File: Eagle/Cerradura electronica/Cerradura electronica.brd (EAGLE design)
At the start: 48.5 x 50 mm, 38 parts, among them IC1 LD117AS50TR, Q1 2N3904, Q2 IRF540NS, U1 ATMEGA328P_TQFP

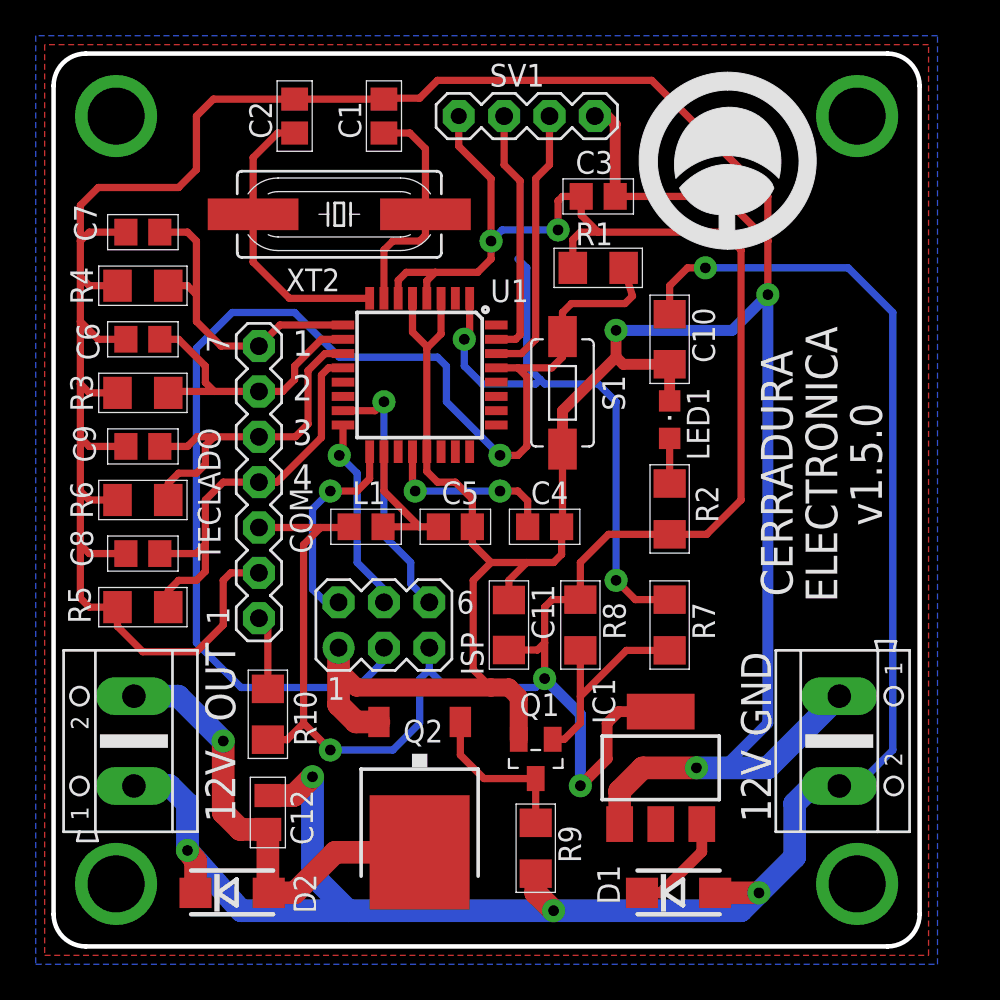
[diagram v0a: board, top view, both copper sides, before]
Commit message: Inicio correciones en PCB
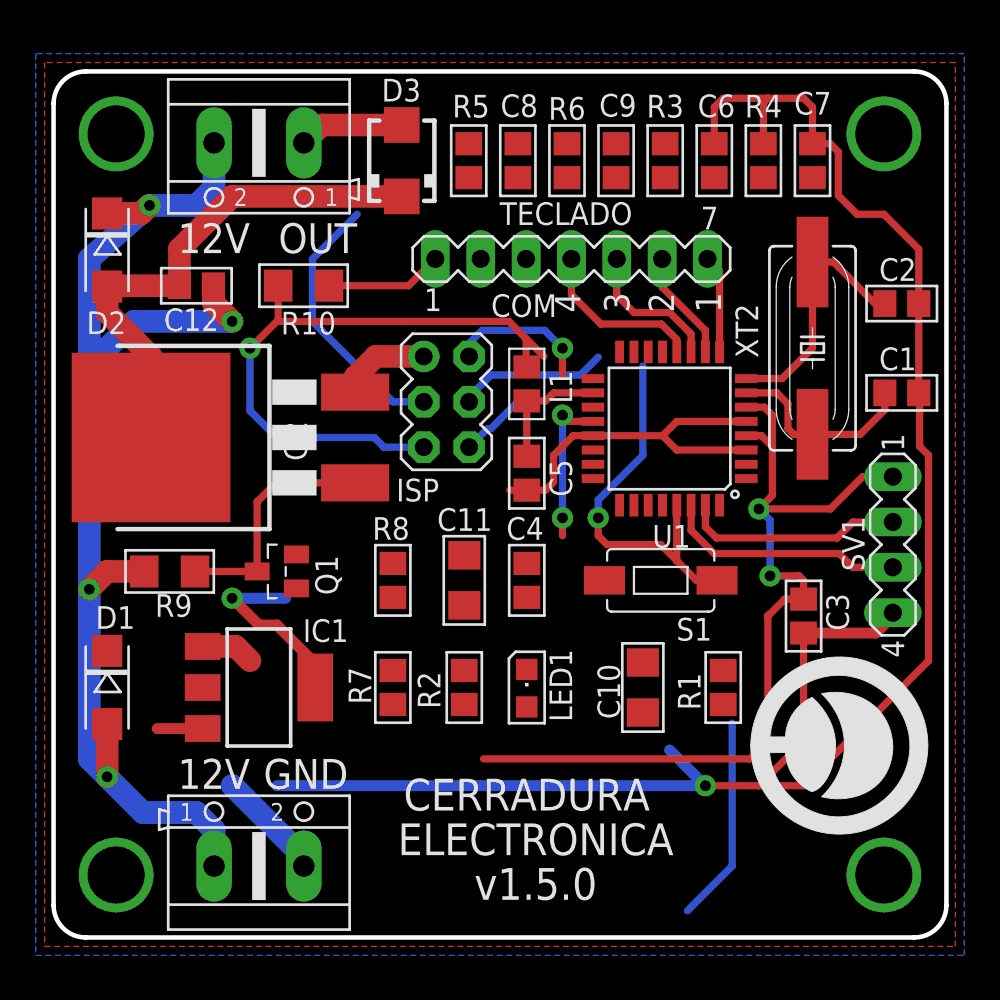
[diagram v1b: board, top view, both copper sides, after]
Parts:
- added D3: MBRA340T3, diode:SMA
- C1, C12, C2, C3, C4, C5, C6, C7, C8, C9: device rcl:C0805 -> CaliBeta-RCL:C0805
- C10, C11: device rcl:C1206 -> CaliBeta-RCL:C1206
- D1, D2: device diode:DO214AC -> CaliBeta-Diodos:DO-214AC
- ISP: value (none) -> CON-ISP; device con-lstb:MA03-2 -> CaliBeta-Conectores:HEADER-M2X3
- L1: device Circuitos-Creativos-RCL:L0805 -> CaliBeta-RCL:L0805
- LED1: value Green -> Rojo; device led:CHIPLED_0805 -> CaliBeta-Diodos:LED0805-ROJO
- MOT, PWR: device con-ptr500:AK500/2 -> CaliBeta-Conectores:AK500-2
- Q1: device transistor:SOT23-BEC -> CaliBeta-Transistores:SOT-23_BEC
- Q2: value IRF540NS -> IRF540N; device Circuitos-Creativos-Transistores:TO-252 -> CaliBeta-Transistores:TO-263
- R1, R2, R3, R4, R5, R6, R7, R8: device rcl:R1206 -> CaliBeta-RCL:R0805
- R10, R9: device rcl:R1206 -> CaliBeta-RCL:R1206
- U1: value ATMEGA328P_TQFP -> (none); device SparkFun-DigitalIC:TQFP32-08 -> CaliBeta-Microcontroladores:TQFP32
- moved C7 37.7 mm to (42.5, 44.0), turned to 90 degrees
- moved D2 36.7 mm to (3.00, 39.0), turned to 270 degrees
- moved C2 35.6 mm to (47.5, 36.0), turned to 0 degrees
- moved R4 35.4 mm to (39.8, 44.0), turned to 90 degrees
- moved MOT 34.2 mm to (11.5, 45.0), turned to 180 degrees
- moved D1 34.0 mm to (3.00, 14.5), turned to 270 degrees
- moved C6 33.5 mm to (37.0, 44.0), turned to 90 degrees
- moved U$1 33.3 mm to (44.0, 11.2), turned to 270 degrees
- moved PWR 33.2 mm to (11.5, 4.50), turned to 0 degrees
- moved C1 32.9 mm to (47.5, 31.0), turned to 0 degrees
- moved R3 32.0 mm to (34.2, 44.0), turned to 90 degrees
- moved SV1 31.6 mm to (47.0, 22.5), turned to 270 degrees
- moved C9 31.0 mm to (31.5, 44.0), turned to 90 degrees
- moved R5 31.0 mm to (23.2, 44.0), turned to 90 degrees
- moved R6 30.4 mm to (28.8, 44.0), turned to 90 degrees
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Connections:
- removed net MOT_ON: C12.2, D2.A, MOT.2, Q2.3
- new net MOT: D3.A, MOT.1
- new net ON: C12.2, D2.A, D3.C, Q2.2
- net +12V: now also D2.K, MOT.2, PWR.1; no longer D2.C, MOT.1, PWR.2
- net GND: now also PWR.2, Q2.3; no longer PWR.1, Q2.2
- net N$3: now also D1.K; no longer D1.C
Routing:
- net GND: track 249.1 -> 138.2 mm, vias 3 -> 1
- net D3: track 34.2 -> 0.00 mm, vias 2 -> 0
- net RST: track 70.4 -> 36.5 mm
- net +12V: track 111.3 -> 81.7 mm, vias 5 -> 4
- net VCC: track 125.3 -> 96.0 mm, vias 5 -> 4
- net ON: track 0.00 -> 29.3 mm
- net MOT_ON: track 25.9 -> 0.00 mm, vias 1 -> 0
- net D8/3: track 23.0 -> 9.64 mm
- net D5/2: track 17.8 -> 5.49 mm
- net N$2: track 12.1 -> 0.00 mm
- net MOSI: track 14.8 -> 3.78 mm, vias 1 -> 0
- net D7/4: track 19.4 -> 8.81 mm
- net D6/1: track 16.3 -> 6.21 mm
- net MOT: track 0.00 -> 5.90 mm
- net N$4: track 9.09 -> 13.5 mm
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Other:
- board size 48.5 x 50 mm -> 50 x 48.5 mm
